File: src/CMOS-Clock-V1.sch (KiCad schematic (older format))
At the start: 102 parts, among them SW1 SW_Push, SW2 SW_Push, SW3 SW_Push, U1 BAS28,215, U10 74AHC86D,118, U11 74HC390D,652, U12 74HC390D,652, U13 MC14511BDR2G, U14 MC14511BDR2G, U15 MC14511BDR2G, U16 MC14511BDR2G, U17 BC846S,125, U18 74LVC1G74DP,125, U19 BC846S,125, U2 7555, U20 BC846S,125, U3 74AHC1G4215, U4 74AHC3G14DP,125, U5 74HC390D,652, U6 74AHC157D,118, U7 74HC27D,653, U8 74LVC1G157, U9 74AHC08D,118

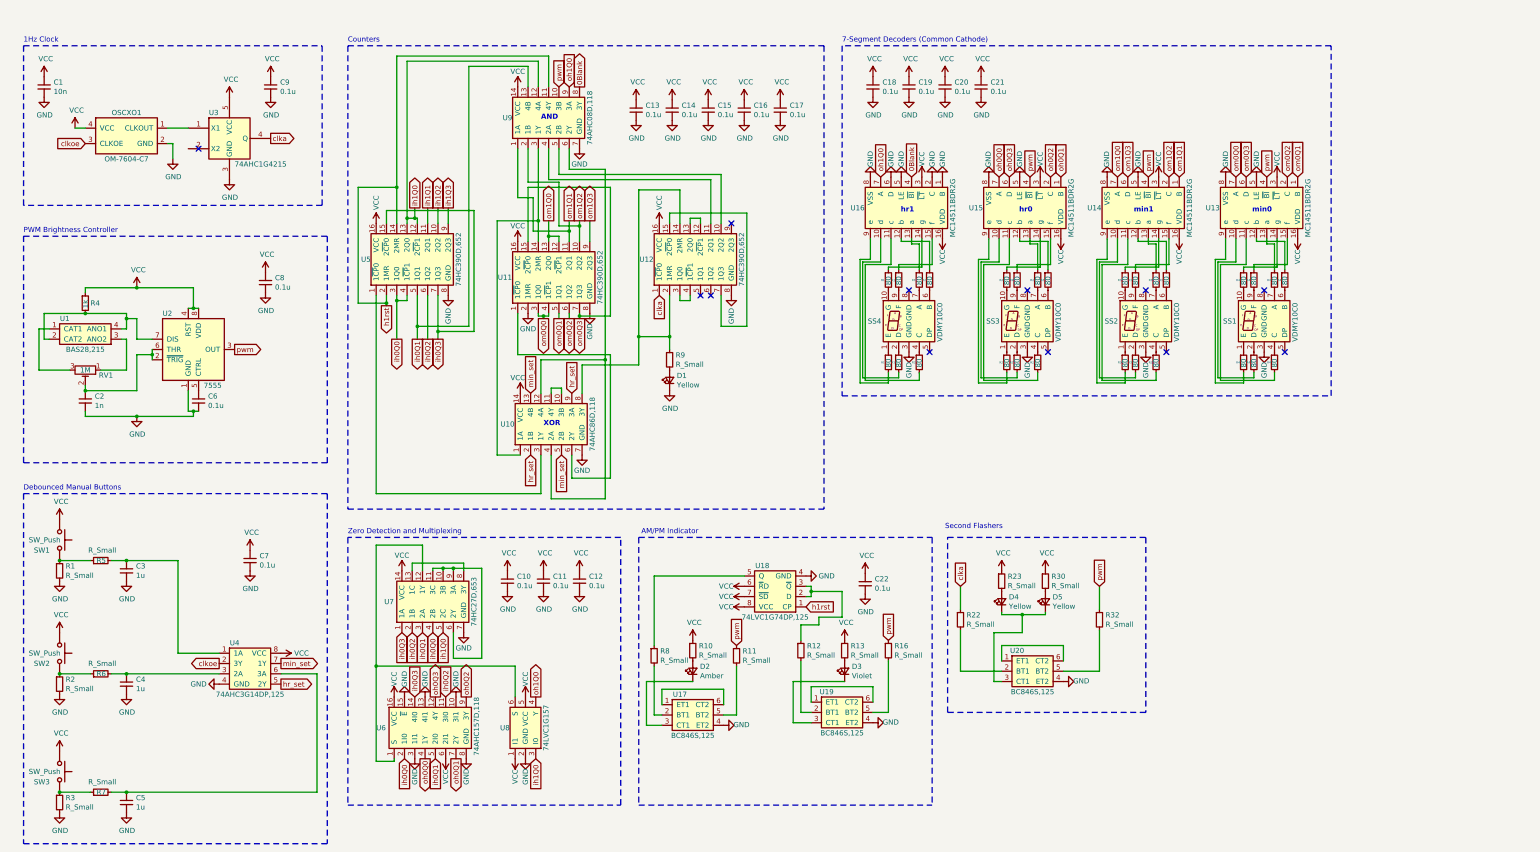
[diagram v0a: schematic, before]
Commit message: Files
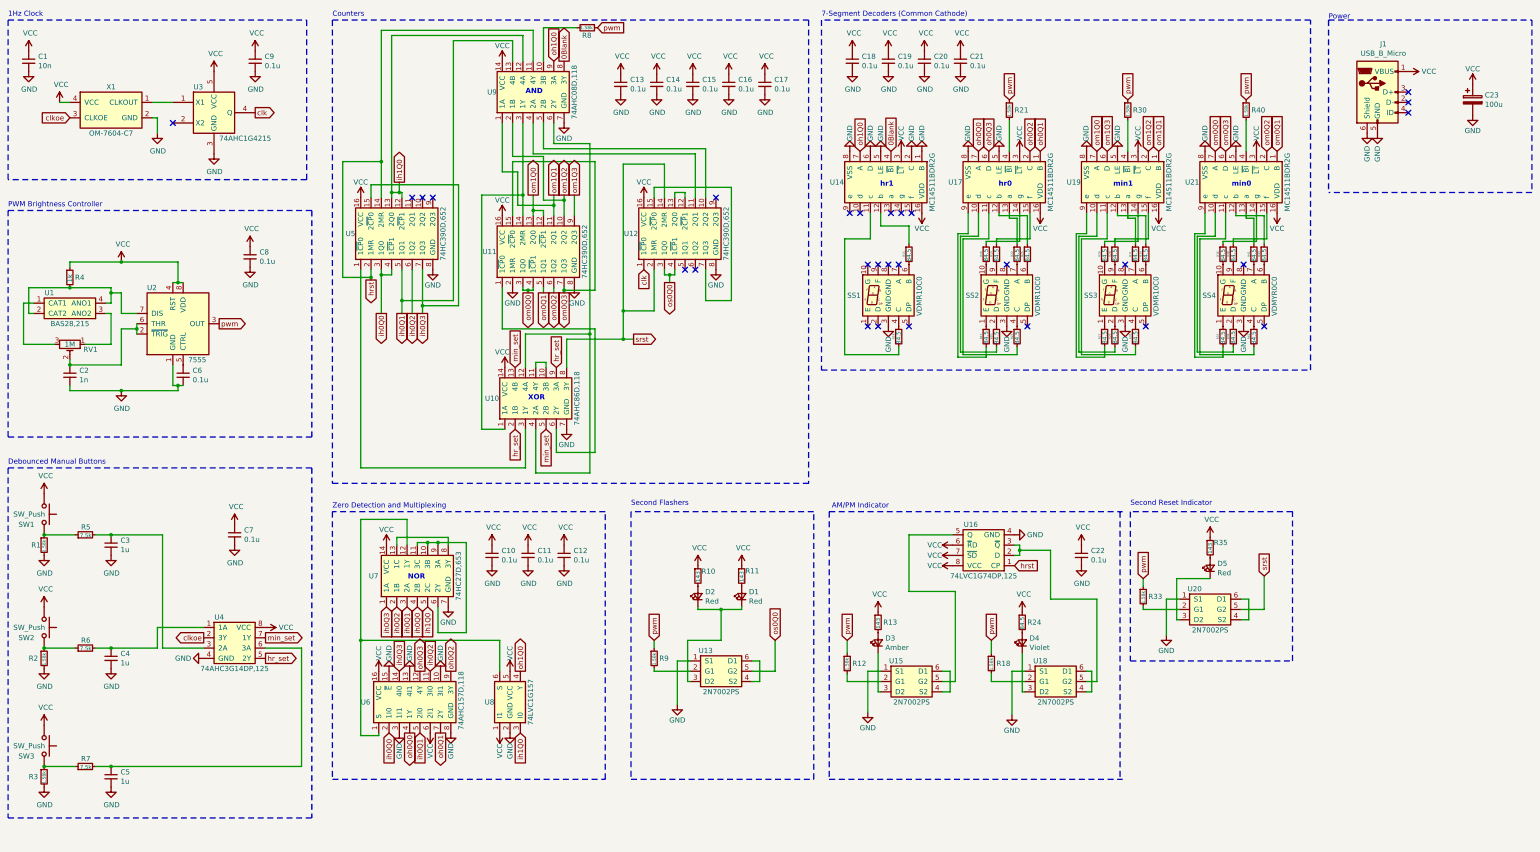
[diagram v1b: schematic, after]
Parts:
- removed D1: Yellow, symbol Device:LED_Small
- removed R11, R16, R22, R32: R_Small, symbol Device:R_Small
- removed R14, R15, R17, R19: 80, symbol Device:R_Small
- removed U17, U19, U20: BC846S,125, symbol CMOS_Clock_V1:BC846S,125
- added C23: 100u, src:865080142007, symbol Device:CP
- added D5: Red, LED_SMD:LED_1206_3216Metric_Pad1.42x1.75mm_HandSolder, symbol Device:LED_Small
- added J1: USB_B_Micro, src:AMPHENOL_10118194-0001LF, symbol Connector:USB_B_Micro
- added R21, R30, R33, R40: 1.58k, Resistor_SMD:R_0805_2012Metric_Pad1.20x1.40mm_HandSolder, symbol Device:R_Small
- added R35: 143, Resistor_SMD:R_1206_3216Metric_Pad1.30x1.75mm_HandSolder, symbol Device:R_Small
- added U13, U15, U18, U20: 2N7002PS, src:SOT363, symbol CMOS_Clock_V1:2N7002PS
- C1, C10, C11, C12, C13, C14, C15, C16, C17, C18, C19, C2, C20, C21, C22, C3, C4, C5, C6, C7, C8, C9: footprint (none) -> Capacitor_SMD:C_0805_2012Metric_Pad1.18x1.45mm_HandSolder
- D1: renamed from D5; value Yellow -> Red; footprint (none) -> LED_SMD:LED_1206_3216Metric_Pad1.42x1.75mm_HandSolder; Part Number (none) -> 5988250107F
- D2: renamed from D4; value Yellow -> Red; footprint (none) -> LED_SMD:LED_1206_3216Metric_Pad1.42x1.75mm_HandSolder; Part Number (none) -> 5988250107F
- D3: renamed from D2; footprint (none) -> LED_SMD:LED_1206_3216Metric_Pad1.42x1.75mm_HandSolder; Part Number (none) -> 5990220007F
- D4: renamed from D3; footprint (none) -> LED_SMD:LED_1206_3216Metric_Pad1.42x1.75mm_HandSolder
- R1, R12, R2, R3, R8, R9: value R_Small -> 1.58k; footprint (none) -> Resistor_SMD:R_0805_2012Metric_Pad1.20x1.40mm_HandSolder
- R10: renamed from R23; value R_Small -> 143; footprint (none) -> Resistor_SMD:R_1206_3216Metric_Pad1.30x1.75mm_HandSolder
- R11: renamed from R30; value R_Small -> 143; footprint (none) -> Resistor_SMD:R_1206_3216Metric_Pad1.30x1.75mm_HandSolder
- R13: renamed from R10; value R_Small -> 143; footprint (none) -> Resistor_SMD:R_1206_3216Metric_Pad1.30x1.75mm_HandSolder; Part Number (none) -> ERJ-8ENF1470V
- R14: renamed from R20; value 80 -> 84.5; footprint (none) -> Resistor_SMD:R_1206_3216Metric_Pad1.30x1.75mm_HandSolder
- R15: renamed from R21; value 80 -> 84.5; footprint (none) -> Resistor_SMD:R_1206_3216Metric_Pad1.30x1.75mm_HandSolder
- R16: renamed from R24; value 80 -> 84.5; footprint (none) -> Resistor_SMD:R_1206_3216Metric_Pad1.30x1.75mm_HandSolder
- R17: renamed from R25; value 80 -> 84.5; footprint (none) -> Resistor_SMD:R_1206_3216Metric_Pad1.30x1.75mm_HandSolder
- R18: value 80 -> 1.58k; footprint (none) -> Resistor_SMD:R_0805_2012Metric_Pad1.20x1.40mm_HandSolder
- R19: renamed from R26; value 80 -> 84.5; footprint (none) -> Resistor_SMD:R_1206_3216Metric_Pad1.30x1.75mm_HandSolder
- R20: renamed from R27; value 80 -> 84.5; footprint (none) -> Resistor_SMD:R_1206_3216Metric_Pad1.30x1.75mm_HandSolder
- R22: renamed from R28; value 80 -> 84.5; footprint (none) -> Resistor_SMD:R_1206_3216Metric_Pad1.30x1.75mm_HandSolder
- R23: renamed from R29; value 80 -> 84.5; footprint (none) -> Resistor_SMD:R_1206_3216Metric_Pad1.30x1.75mm_HandSolder
- R24: renamed from R13; value R_Small -> 84.5; footprint (none) -> Resistor_SMD:R_1206_3216Metric_Pad1.30x1.75mm_HandSolder; Part Number (none) -> ERJ-8ENF1470V
- R25: renamed from R31; value 80 -> 84.5; footprint (none) -> Resistor_SMD:R_1206_3216Metric_Pad1.30x1.75mm_HandSolder
- R26: renamed from R33; value 80 -> 84.5; footprint (none) -> Resistor_SMD:R_1206_3216Metric_Pad1.30x1.75mm_HandSolder
- R27: renamed from R34; value 80 -> 84.5; footprint (none) -> Resistor_SMD:R_1206_3216Metric_Pad1.30x1.75mm_HandSolder
- R28: renamed from R35; value 80 -> 84.5; footprint (none) -> Resistor_SMD:R_1206_3216Metric_Pad1.30x1.75mm_HandSolder
- R29: renamed from R36; value 80 -> 84.5; footprint (none) -> Resistor_SMD:R_1206_3216Metric_Pad1.30x1.75mm_HandSolder
- R31: renamed from R37; value 80 -> 84.5; footprint (none) -> Resistor_SMD:R_1206_3216Metric_Pad1.30x1.75mm_HandSolder
- R32: renamed from R38; value 80 -> 84.5; footprint (none) -> Resistor_SMD:R_1206_3216Metric_Pad1.30x1.75mm_HandSolder
- R34: renamed from R39; value 80 -> 84.5; footprint (none) -> Resistor_SMD:R_1206_3216Metric_Pad1.30x1.75mm_HandSolder
- R36: renamed from R40; value 80 -> 84.5; footprint (none) -> Resistor_SMD:R_1206_3216Metric_Pad1.30x1.75mm_HandSolder
- R37: renamed from R41; value 80 -> 84.5; footprint (none) -> Resistor_SMD:R_1206_3216Metric_Pad1.30x1.75mm_HandSolder
- R38: renamed from R42; value 80 -> 84.5; footprint (none) -> Resistor_SMD:R_1206_3216Metric_Pad1.30x1.75mm_HandSolder
- R39: renamed from R43; value 80 -> 84.5; footprint (none) -> Resistor_SMD:R_1206_3216Metric_Pad1.30x1.75mm_HandSolder
- R4: footprint (none) -> Resistor_SMD:R_0805_2012Metric_Pad1.20x1.40mm_HandSolder
- R41: renamed from R44; value 80 -> 84.5; footprint (none) -> Resistor_SMD:R_1206_3216Metric_Pad1.30x1.75mm_HandSolder
- R42: renamed from R45; value 80 -> 84.5; footprint (none) -> Resistor_SMD:R_1206_3216Metric_Pad1.30x1.75mm_HandSolder
- R43: renamed from R46; value 80 -> 84.5; footprint (none) -> Resistor_SMD:R_1206_3216Metric_Pad1.30x1.75mm_HandSolder
- R5, R6, R7: value R_Small -> 7.5k; footprint (none) -> Resistor_SMD:R_0805_2012Metric_Pad1.20x1.40mm_HandSolder
- RV1: footprint (none) -> src:TRIM_TC33X-2-105E
- SS1: renamed from SS4; value VDMY10C0 -> VDMR10C0; footprint (none) -> src:VDMR10C0
- SS2: renamed from SS3; value VDMY10C0 -> VDMR10C0; footprint (none) -> src:VDMR10C0
- SS3: renamed from SS2; value VDMY10C0 -> VDMR10C0; footprint (none) -> src:VDMR10C0
- SS4: renamed from SS1; value VDMY10C0 -> VDMYR0C0; footprint (none) -> src:VDMR10C0
- SW1, SW2, SW3: footprint (none) -> src:PTS 647 SK38 SMTR2 LFS
- U1: footprint (none) -> src:SOT143(B)
- U10, U7, U9: footprint (none) -> src:SOT108-1
- U11, U12, U5, U6: footprint (none) -> src:SOT109-1
- U14: renamed from U16; footprint (none) -> src:SOT109-1
- U16: renamed from U18; footprint (none) -> src:SOT505-2
- U17: renamed from U15; footprint (none) -> src:SOT109-1
- U19: renamed from U14; footprint (none) -> src:SOT109-1
- U2: footprint (none) -> src:ICM7555
- U21: renamed from U13; footprint (none) -> src:SOT109-1
- U3: footprint Package_TO_SOT_SMD:SOT-353_SC-70-5 -> src:74AHC1G4215
- U4: footprint (none) -> src:SOT505-2
- U8: footprint (none) -> src:SOT457
- X1: renamed from OSCXO1; footprint (none) -> src:OSC_OM-7604-C7
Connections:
- net GND: now also C23.2, J1.5 (GND), J1.6 (Shield), U13.1 (S1), U15.1 (S1), U18.1 (S1), U20.1 (S1)
- net VCC: now also C23.1, J1.1 (VBUS), R35.1
- net pwm: now also R12.1, R18.1, R8.1, R9.1, R21.1, R30.1, R33.1, R40.1; no longer U17.4 (~BI~), U19.4 (~BI~), U21.4 (~BI~), U9.10 (3B)
- net srst: now reaches U10.8 (3Y), U12.14 (2MR), U12.2 (1MR)
- net srst: now also U20.5 (G2); no longer R9.1
- net os0Q0: now reaches U12.3 (1Q0), U12.4 (1~CP~1)
- net os0Q0: now also U13.5 (G2)
- net at C3.1, R5.2: now also U4.3 (2A); no longer U4.1 (1A)
- net at C4.1, R6.2: now also U4.1 (1A); no longer U4.3 (2A)
- net at R18.2: now also U18.2 (G1); no longer U14.10 (d)
- net at SS1.2 (D): no longer R18.1
- net at U16.2 (D), U16.3 (~Q): now also U18.5 (G2); no longer R12.1
- net at U16.5 (Q): now also U15.5 (G2); no longer R8.1
- net at R8.2: now also U9.10 (3B)
- net at D3.1 (K): now also U15.3 (D2)
- net at R12.2: now also U15.2 (G1)
- net at D4.1 (K): now also U18.3 (D2)
- net at D1.1 (K), D2.1 (K): now also U13.3 (D2)
- net at R9.2: now also U13.2 (G1)
- net clka renamed clk
- net h1rst renamed hrst
- net ih1Q1: no longer names the net of U5.11 (2Q1)
- net ih1Q2: no longer names the net of U5.10 (2Q2)
- net ih1Q3: no longer names the net of U5.9 (2Q3)
- new net: D5.1 (K), U20.3 (D2)
- new net: D5.2 (A), R35.2
- new net: R33.2, U20.2 (G1)
- new net: U20.4 (S2), U20.6 (D1)
- new net: R40.2, U21.4 (~BI~)
- new net: R21.2, U17.4 (~BI~)
- new net: R30.2, U19.4 (~BI~)
- new net: U15.4 (S2), U15.6 (D1)
- new net: U18.4 (S2), U18.6 (D1)
- new net: U13.4 (S2), U13.6 (D1)
- no-connect marks 12 -> 28
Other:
- note added: "NOR"
- note added: "Power"
- note added: "Second Reset Indicator"
- moved on the sheet: C1, C10, C11, C12, C13, C14, C15, C16, C17, C18, C19, C2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
